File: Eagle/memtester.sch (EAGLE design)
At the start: 4 parts

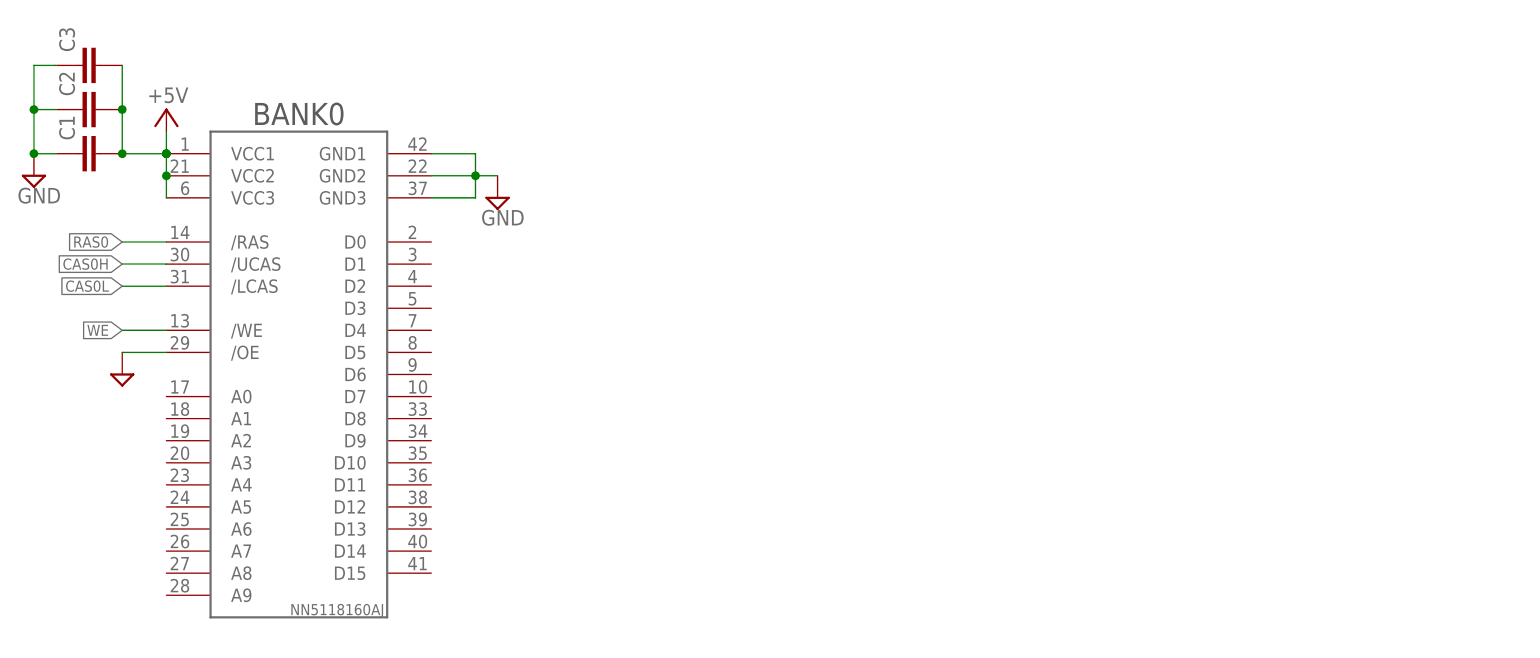
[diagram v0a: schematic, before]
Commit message: Memtester: part work backup
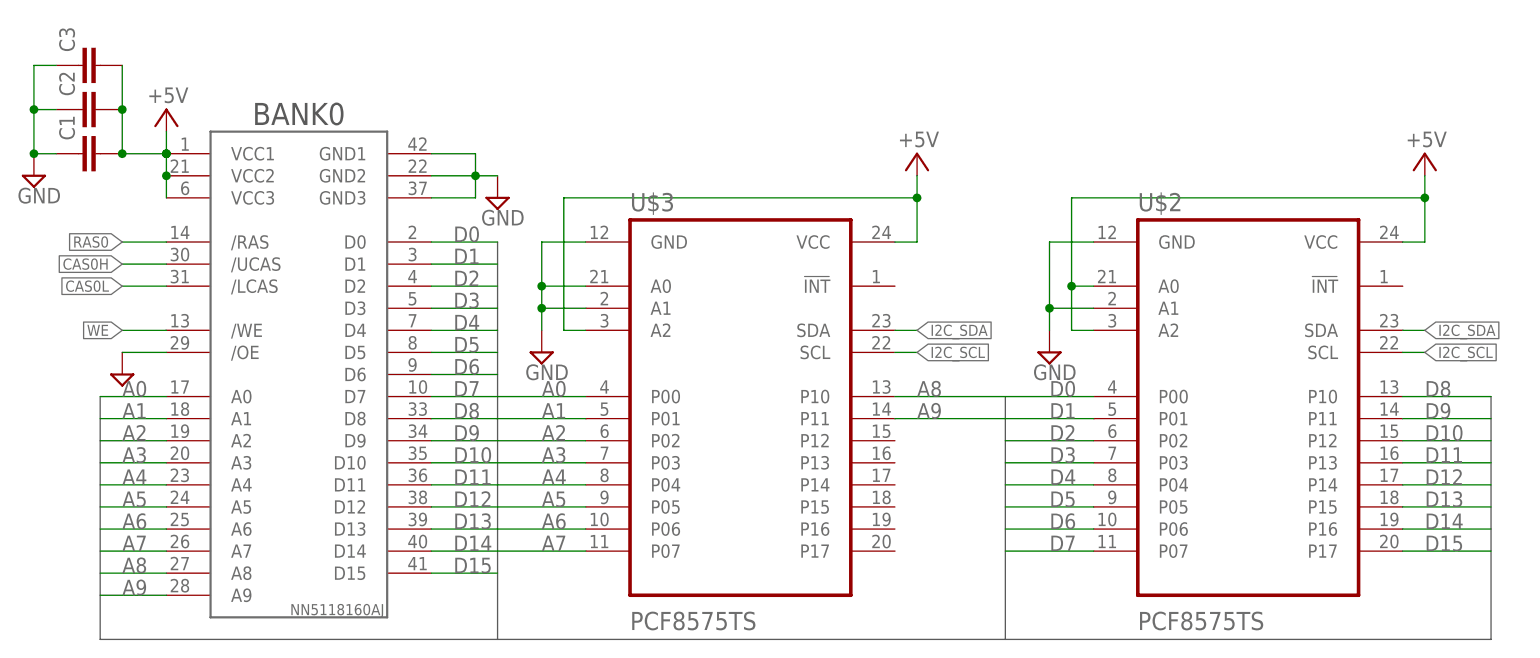
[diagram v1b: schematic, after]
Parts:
- added U$2, U$3: PCF8575TS, PCF8575TS:PCF8575TS
- U$1: value NN5118160AJ -> NN5118160AJSOCKET; device AtariST:NN5118160AJ -> memory:NN5118160AJSOCKET
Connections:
- new net A0: U$1.A0, U$3.P00
- new net A1: U$1.A1, U$3.P01
- new net A2: U$1.A2, U$3.P02
- new net A3: U$1.A3, U$3.P03
- new net A4: U$1.A4, U$3.P04
- new net A5: U$1.A5, U$3.P05
- new net A6: U$1.A6, U$3.P06
- new net A7: U$1.A7, U$3.P07
- new net A8: U$1.A8, U$3.P10
- new net A9: U$1.A9, U$3.P11
- new net D0: U$1.D0, U$2.P00
- new net D1: U$1.D1, U$2.P01
- new net D10: U$1.D10, U$2.P12
- new net D11: U$1.D11, U$2.P13
- new net D12: U$1.D12, U$2.P14
- new net D13: U$1.D13, U$2.P15
- new net D14: U$1.D14, U$2.P16
- new net D15: U$1.D15, U$2.P17
- new net D2: U$1.D2, U$2.P02
- new net D3: U$1.D3, U$2.P03
- new net D4: U$1.D4, U$2.P04
- new net D5: U$1.D5, U$2.P05
- new net D6: U$1.D6, U$2.P06
- new net D7: U$1.D7, U$2.P07
- new net D8: U$1.D8, U$2.P10
- new net D9: U$1.D9, U$2.P11
- new net I2C_SCL: U$2.SCL, U$3.SCL
- new net I2C_SDA: U$2.SDA, U$3.SDA
- net +5V: now also U$2.A0, U$2.A2, U$2.VCC, U$3.A2, U$3.VCC
- net GND: now also U$2.A1, U$2.GND, U$3.A0, U$3.A1, U$3.GND
